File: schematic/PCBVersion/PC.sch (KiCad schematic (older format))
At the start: 8 parts

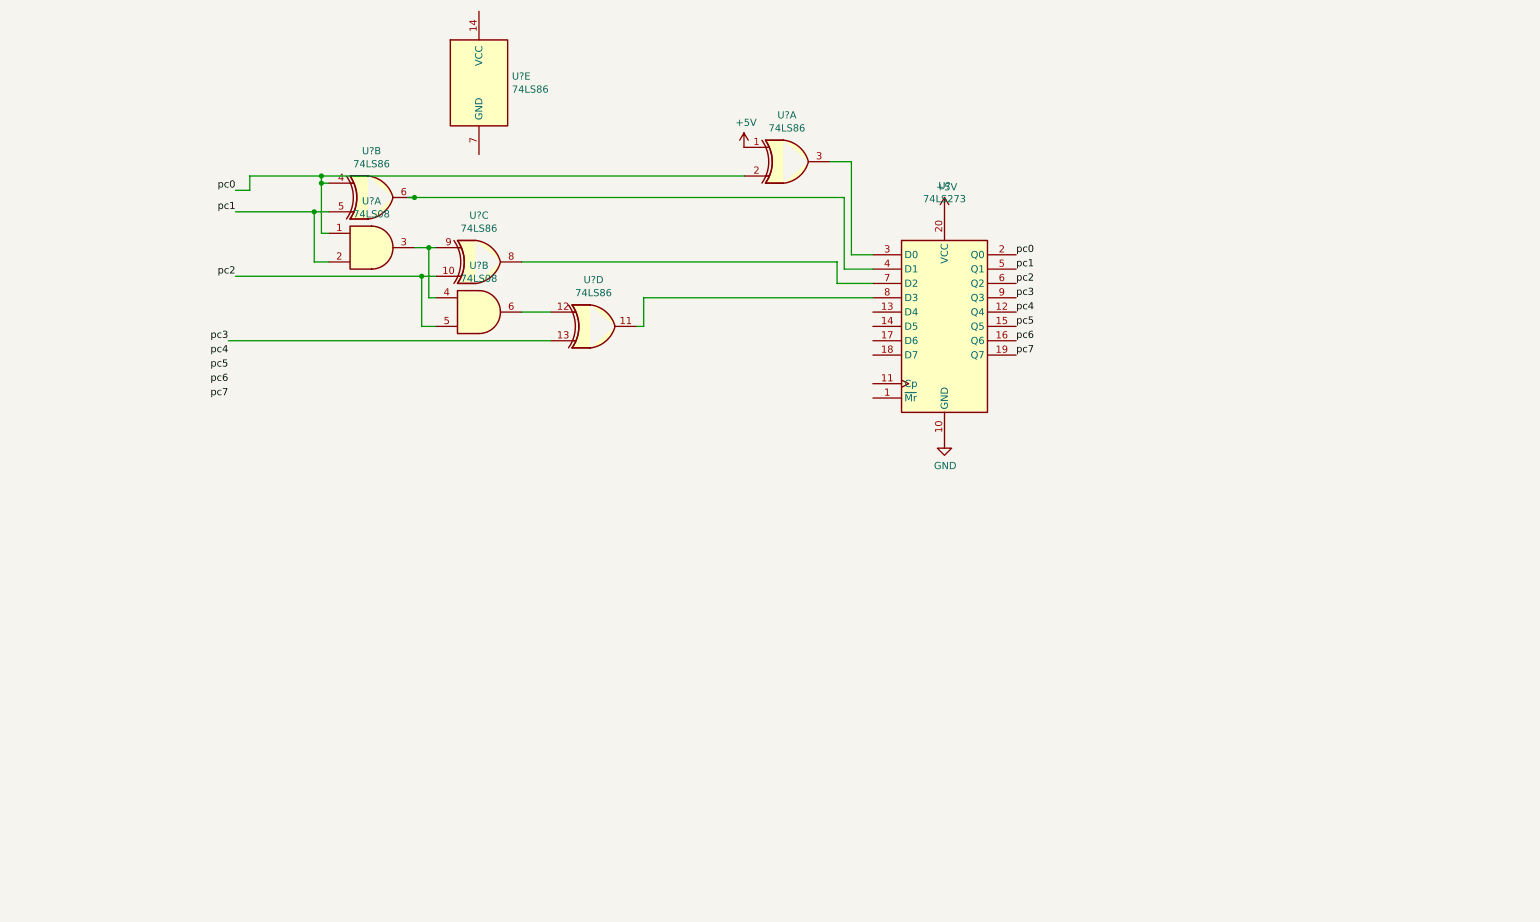
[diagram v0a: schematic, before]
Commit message: pcbVersion: kinda done
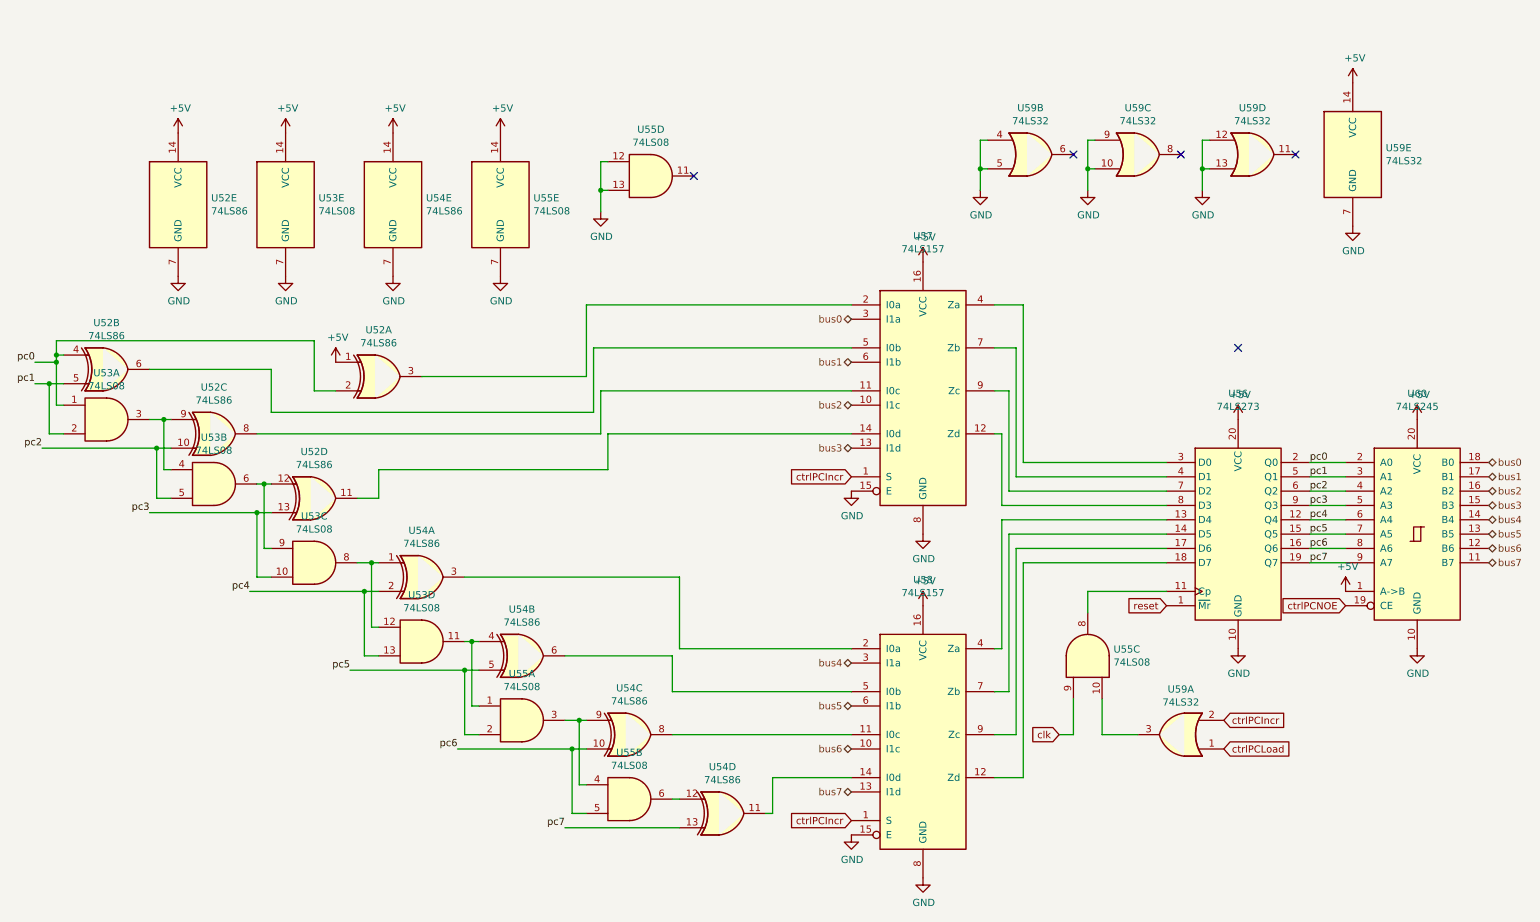
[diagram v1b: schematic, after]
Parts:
- added unit 3 of U53
- added unit 4 of U53
- added unit 5 of U53
- added U54: 74LS86, Package_DIP:DIP-14_W7.62mm, symbol 74xx:74LS86
- added U55: 74LS08, Package_DIP:DIP-14_W7.62mm, symbol 74xx:74LS08
- added U57, U58: 74LS157, Package_DIP:DIP-16_W7.62mm, symbol 74xx:74LS157
- added U59: 74LS32, Package_DIP:DIP-14_W7.62mm, symbol 74xx:74LS32
- added U60: 74LS245, Package_DIP:DIP-20_W7.62mm, symbol 74xx:74LS245
- U52, U53: renamed from U?; footprint (none) -> Package_DIP:DIP-14_W7.62mm
- U56: renamed from U?; footprint (none) -> Package_DIP:DIP-20_W7.62mm
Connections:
- net labels added: bus0, bus1, bus2, bus3, bus4, bus5, bus6, bus7, clk, ctrlPCIncr, ctrlPCLoad, ctrlPCNOE, reset
- wire segments 35 -> 135
- no-connect marks 0 -> 5
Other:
- moved on the sheet: U52A, U52B, U52C, U52D, U52E, U53A, U53B, U56
